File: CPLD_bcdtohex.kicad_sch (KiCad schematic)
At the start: 26 parts, among them IC1 ATF750C-10PU, J1 Conn_01x06, J2 Conn_01x02

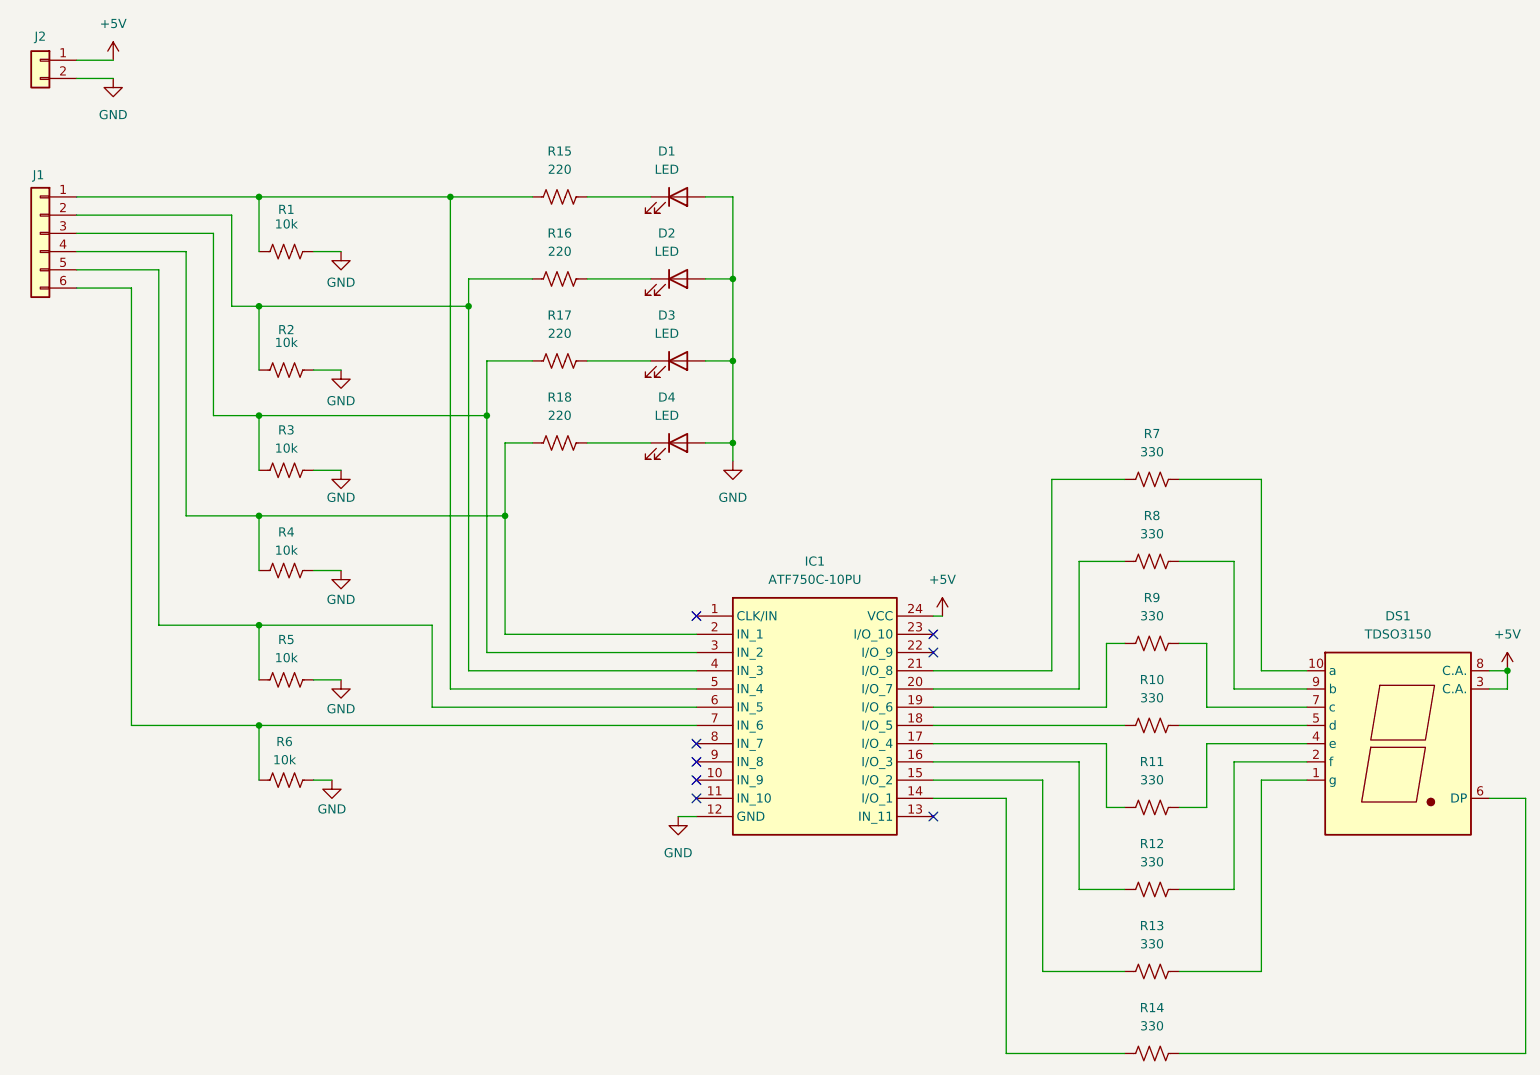
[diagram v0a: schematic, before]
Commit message: Initial commit
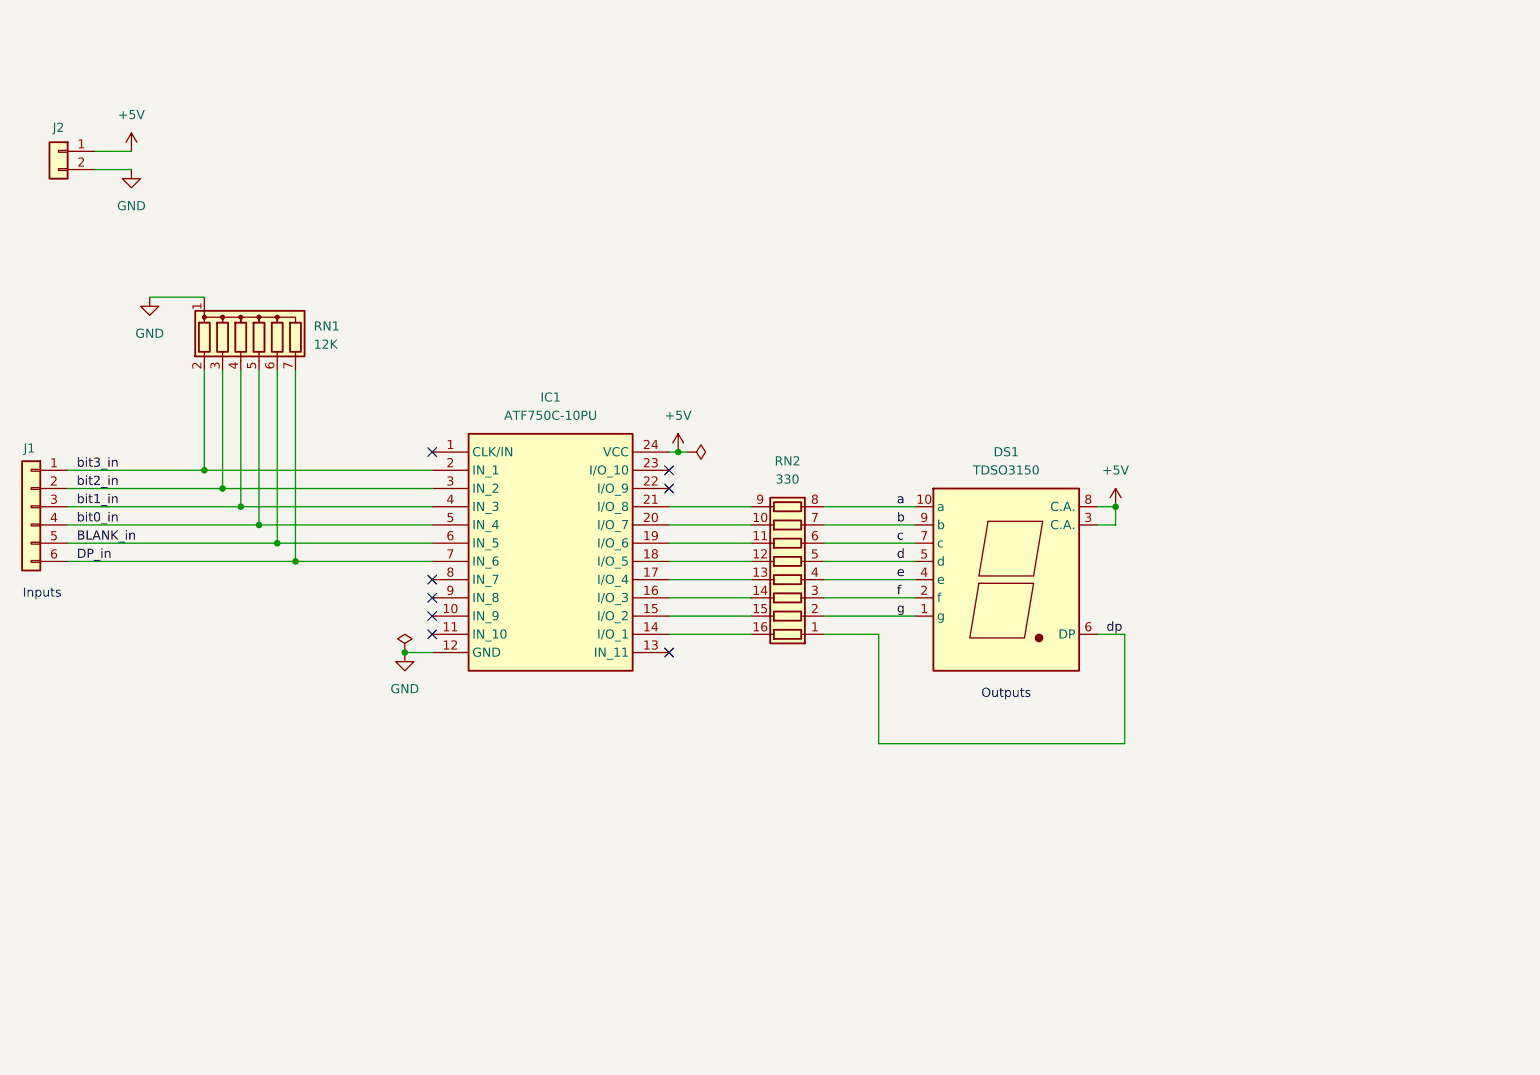
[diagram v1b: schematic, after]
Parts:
- removed D1, D2, D3, D4: LED, LED_THT:LED_D5.0mm, symbol Device:LED
- removed R1, R2, R3, R4, R5, R6: 10k, Resistor_THT:R_Axial_DIN0204_L3.6mm_D1.6mm_P5.08mm_Horizontal, symbol Device:R_US
- removed R10, R11, R12, R13, R14, R7, R8, R9: 330, Resistor_THT:R_Axial_DIN0204_L3.6mm_D1.6mm_P5.08mm_Horizontal, symbol Device:R_US
- removed R15, R16, R17, R18: 220, Resistor_THT:R_Axial_DIN0204_L3.6mm_D1.6mm_P5.08mm_Horizontal, symbol Device:R_US
- added RN1: 12K, Resistor_THT:R_Array_SIP7, symbol Device:R_Network06
- added RN2: 330, Package_DIP:DIP-16_W7.62mm, symbol Device:R_Pack08
- IC1: footprint Package_DIP:DIP-24_W15.24mm -> Package_DIP:DIP-24_W10.16mm
- J1: footprint (none) -> Connector_PinHeader_2.54mm:PinHeader_1x06_P2.54mm_Vertical
- J2: footprint (none) -> Connector_PinHeader_2.54mm:PinHeader_1x02_P2.54mm_Vertical
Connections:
- net GND: now also RN1.1 (common)
- net bit1_in: now reaches IC1.4 (IN_3)
- net bit1_in: now also J1.3 (Pin_3), RN1.4 (R3); no longer J1.2 (Pin_2)
- net at IC1.21 (I/O_8): now also RN2.9 (R8.2)
- net a: now reaches DS1.10 (a)
- net a: now also RN2.8 (R8.1)
- net BLANK_in: now reaches IC1.6 (IN_5), J1.5 (Pin_5)
- net BLANK_in: now also RN1.6 (R5)
- net bit0_in: now reaches J1.4 (Pin_4)
- net bit0_in: now also IC1.5 (IN_4), RN1.5 (R4); no longer IC1.2 (IN_1)
- net g: now reaches DS1.1 (g)
- net g: now also RN2.2 (R2.1)
- net f: now reaches DS1.2 (f)
- net f: now also RN2.3 (R3.1)
- net e: now reaches DS1.4 (e)
- net e: now also RN2.4 (R4.1)
- net d: now reaches DS1.5 (d)
- net d: now also RN2.5 (R5.1)
- net dp: now reaches DS1.6 (DP)
- net dp: now also RN2.1 (R1.1)
- net c: now reaches DS1.7 (c)
- net c: now also RN2.6 (R6.1)
- net b: now reaches DS1.9 (b)
- net b: now also RN2.7 (R7.1)
- net at IC1.18 (I/O_5): now also RN2.12 (R5.2)
- net at IC1.14 (I/O_1): now also RN2.16 (R1.2)
- net at IC1.15 (I/O_2): now also RN2.15 (R2.2)
- net at IC1.16 (I/O_3): now also RN2.14 (R3.2)
- net at IC1.17 (I/O_4): now also RN2.13 (R4.2)
- net at IC1.19 (I/O_6): now also RN2.11 (R6.2)
- net at IC1.20 (I/O_7): now also RN2.10 (R7.2)
- net bit2_in: now reaches IC1.3 (IN_2)
- net bit2_in: now also J1.2 (Pin_2), RN1.3 (R2); no longer J1.3 (Pin_3)
- net bit3_in: now reaches J1.1 (Pin_1)
- net bit3_in: now also IC1.2 (IN_1), RN1.2 (R1); no longer IC1.5 (IN_4)
- net DP_in: now reaches IC1.7 (IN_6), J1.6 (Pin_6)
- net DP_in: now also RN1.7 (R6)
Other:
- note added: "Inputs"
- note added: "Outputs"
- moved on the sheet: DS1, IC1, J1, J2
